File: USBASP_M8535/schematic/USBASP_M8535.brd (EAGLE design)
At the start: 81.3 x 47 mm, 74 parts, among them IC1 MEGA8535, J1 0, J2 0, Q1 12MHz, T1 BC847, T2 BC847, T3 BC847, T4 BC847, T5 BC847, X1 USB_B, X2 MCU_PROGRAMMING, X3 DEVICE_ISP, X4 DEVICE_JTAG_ISP

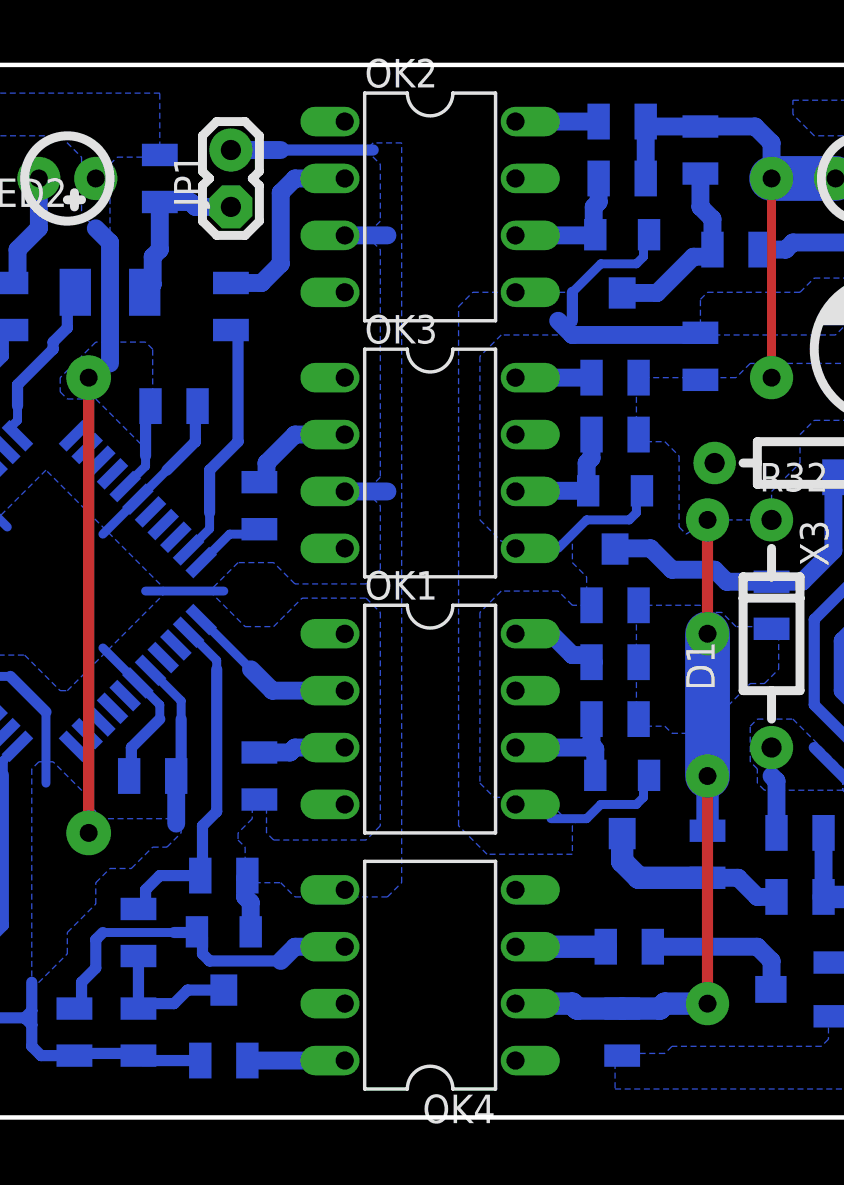
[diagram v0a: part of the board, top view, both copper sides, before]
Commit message: Some level converter values were changed for improve data transfer speed
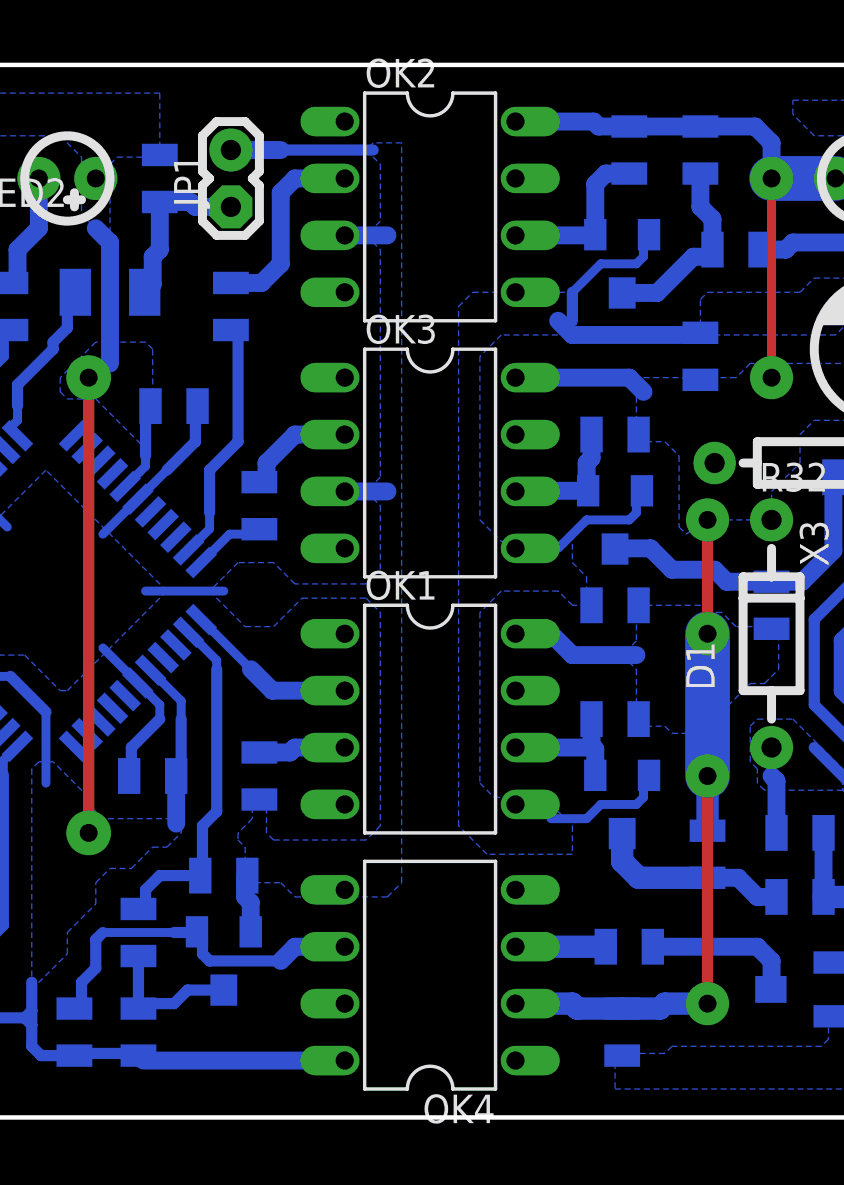
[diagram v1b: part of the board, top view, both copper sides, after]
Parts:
- removed R11, R16, R21, R29: 1K0, __MyCommonLib1:RSMD_0805
- R10, R15, R20, R28: value 4K7 -> 1K0
- R13, R18, R23, R26: value 1K0 -> 240R
- moved R14 1.31 mm to (50.8, 43.2), turned to 270 degrees
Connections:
- removed net N$10: OK1.8, R11.PAD_1
- removed net N$17: OK2.8, R16.PAD_1
- removed net N$23: OK3.8, R21.PAD_1
- removed net N$34: OK4.8, R29.PAD_1
- net +5V_USB: now also OK4.8; no longer R29.PAD_0
- net D_VCC: now also OK1.8, OK2.8, OK3.8; no longer R11.PAD_0, R16.PAD_0, R21.PAD_0
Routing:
- net D_VCC: track 54.8 -> 69.9 mm
- net +5V_USB: track 80.4 -> 86.8 mm
- net N$34: track 4.35 -> 0.00 mm
- net N$10: track 4.12 -> 0.00 mm
- net N$17: track 3.71 -> 0.00 mm
- net N$23: track 3.40 -> 0.00 mm
- net N$18: track 6.21 -> 7.55 mm

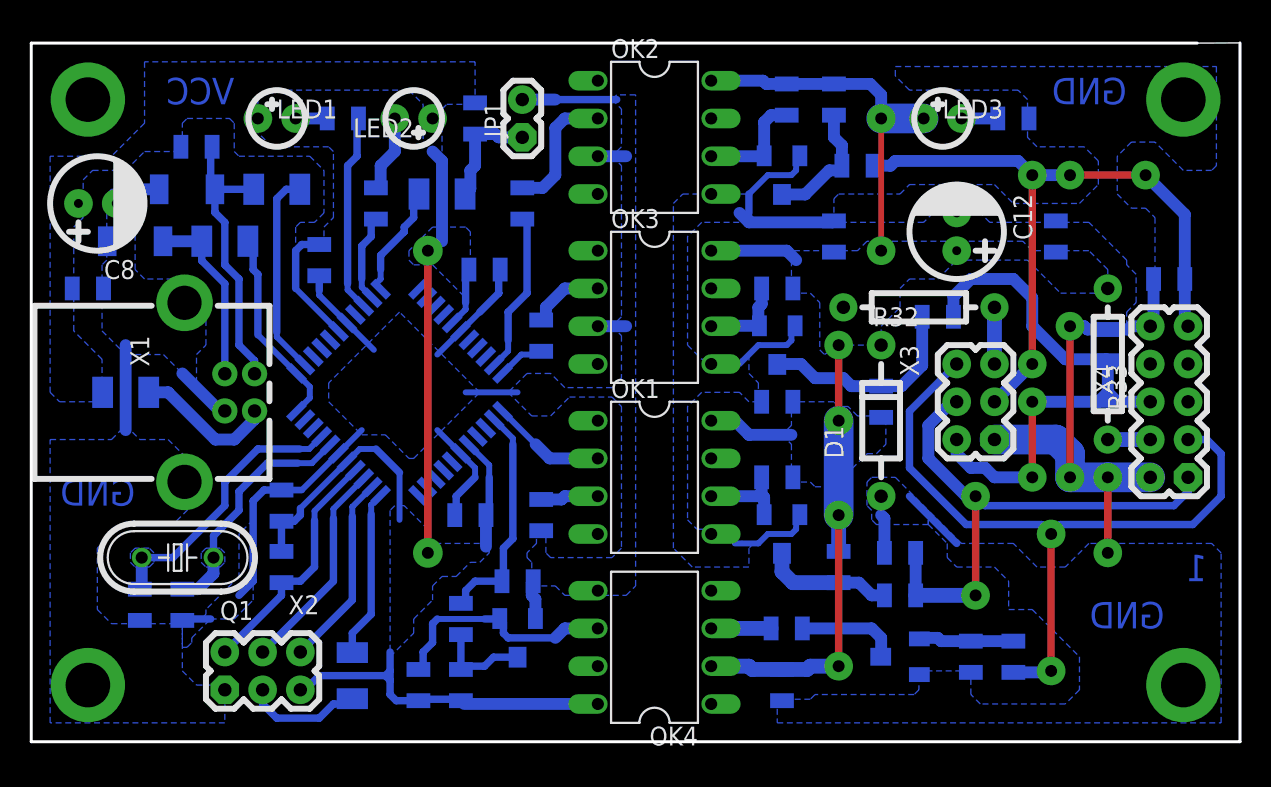
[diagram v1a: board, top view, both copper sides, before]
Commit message: Change again some element valus for correct working on high SCK speed. Remove jumper and add switch for low/high speed selection
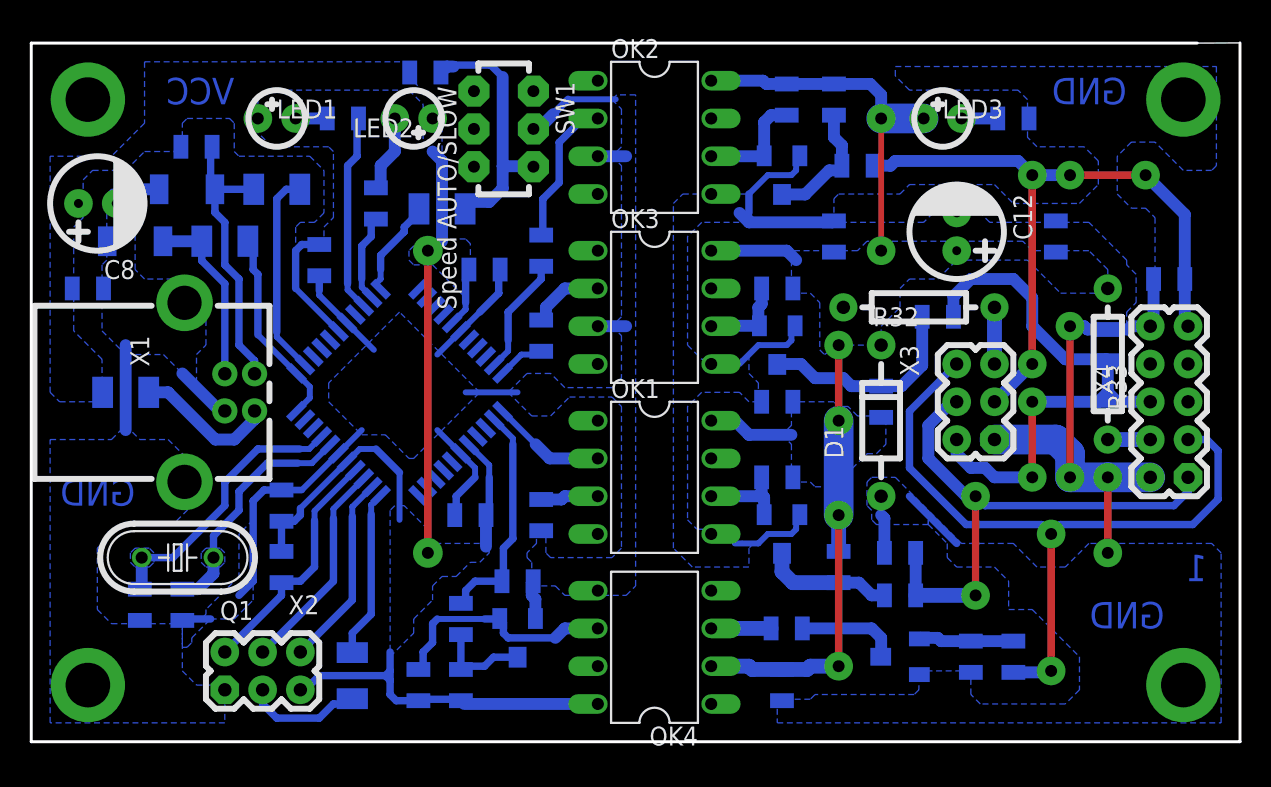
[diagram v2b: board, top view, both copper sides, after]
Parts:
- removed JP1: SLOW_SCK, __MyCommonLib1:PIN2X1_2.54MM
- added SW1: Speed AUTO/SLOW, __MyCommonLib1:SWITCH_DOUBLE_2.54X4.0MM
- moved R7 4.55 mm to (26.5, 45.0), turned to 180 degrees
- moved R18 3.42 mm to (34.3, 33.0)
- moved R8 1.00 mm to (27.6, 35.8)
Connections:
- removed net N$12: JP1.1, R7.PAD_1, R8.PAD_1
- new net N$10: R7.PAD_1, R8.PAD_1, SW1.POS_B2
- net GND: now also SW1.CENTER2; no longer JP1.2
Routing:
- net N$10: track 0.00 -> 17.4 mm
- net N$12: track 7.57 -> 0.00 mm
- net T_MOSI: track 10.9 -> 7.95 mm
- net N$20: track 8.87 -> 10.00 mm
